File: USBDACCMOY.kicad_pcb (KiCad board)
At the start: 2 copper layers, 49.6 x 77.8 mm, 54 parts, among them CON1 GND_CONNECTORSMD, IC1 OPA2134P, J1 USB, Q1 12MHz, U1 NMA0512SC, U2 PCM2707C

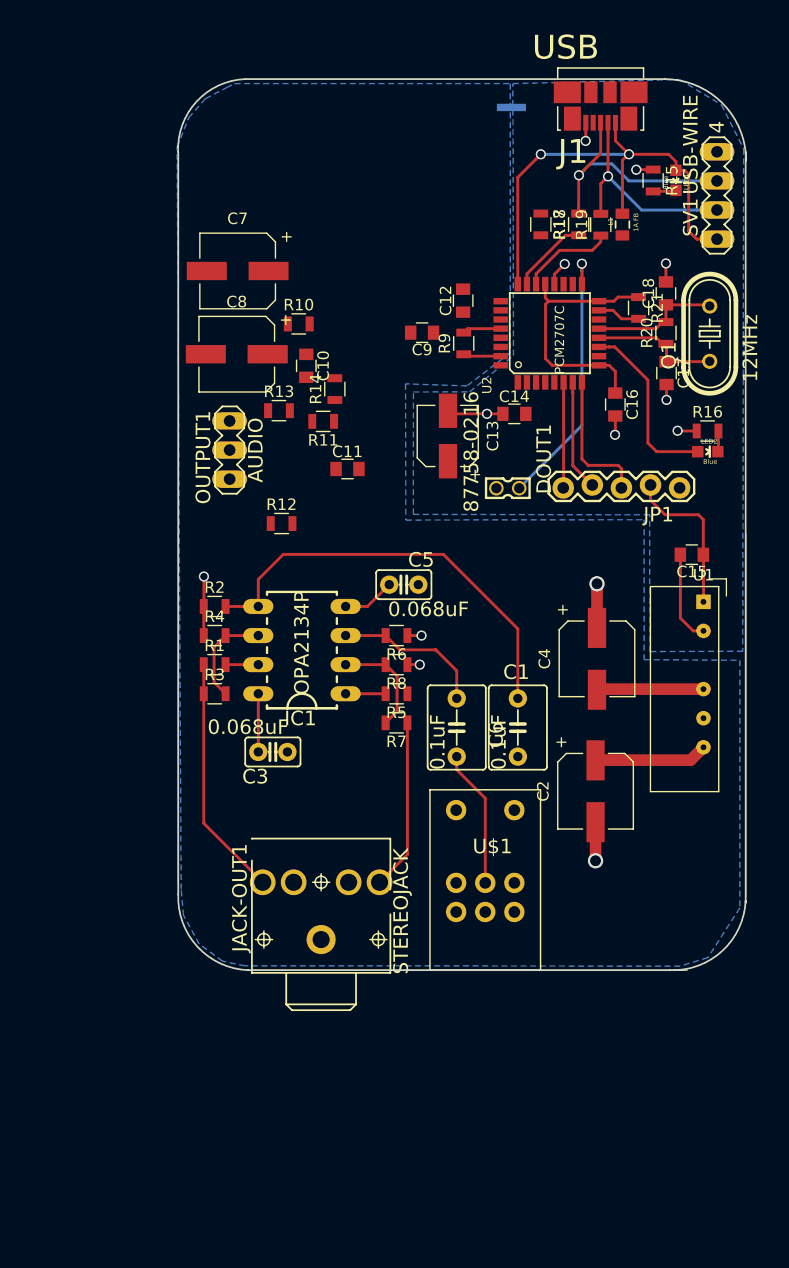
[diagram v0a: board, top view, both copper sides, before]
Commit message: Updated Design Files
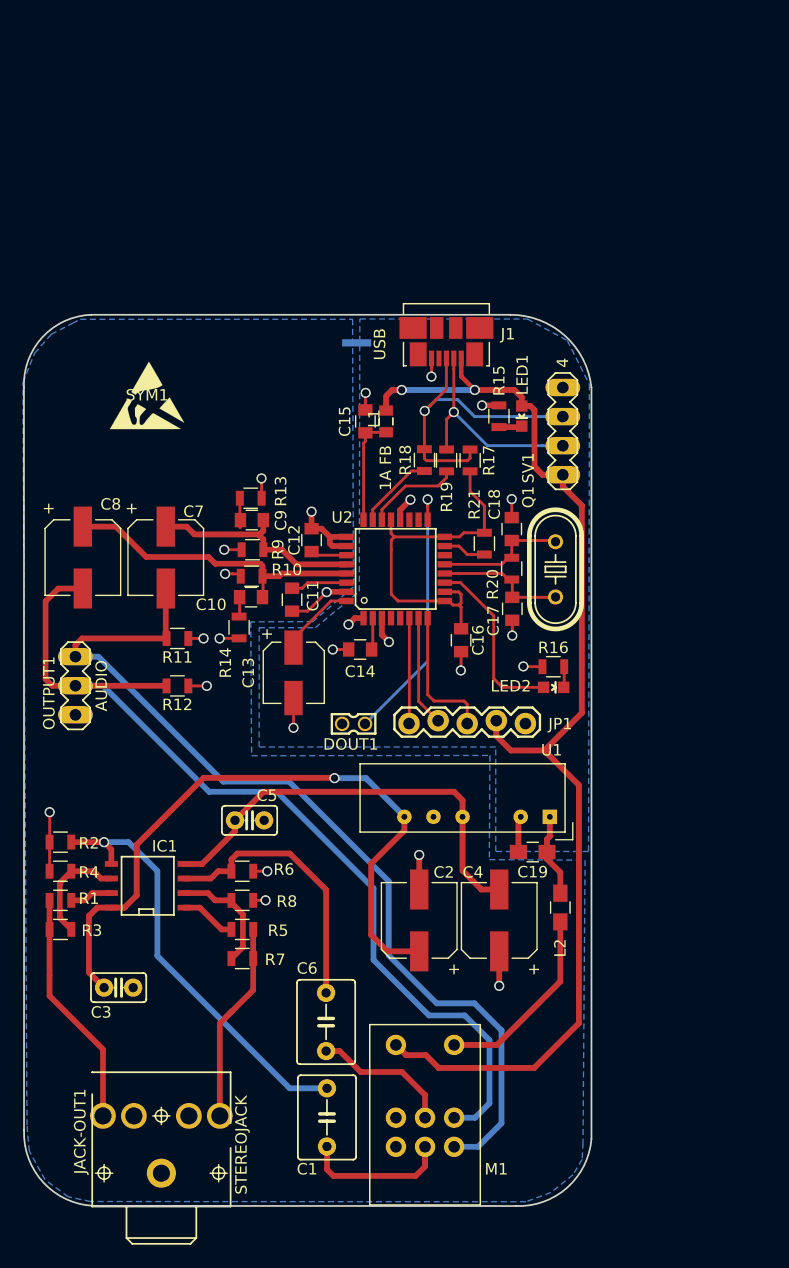
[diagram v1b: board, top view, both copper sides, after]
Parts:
- removed U$1: ~, CMOY:AUDIO-POTS_ALPS_RK0971221Z0X
- added C19: C, Capacitors_SMD:C_0805_HandSoldering, F.Cu at (145.9, 121.4)
- added L2: L, Capacitors_SMD:C_0805_HandSoldering, F.Cu at (148.3, 126.3)
- added M1: AUDIO-POTS_ALPS_RK0971221Z05, PCM2707:AUDIO-POTS_ALPS_RK0971221Z0X, F.Cu at (136.5, 144.6)
- added SYM1: SYM_ESD_Small, Symbols:ESD-Logo_6.6x6mm_SilkScreen, F.Cu at (112.3, 81.5)
- IC1: footprint CMOY:DIL-8 -> SMD_Packages:SOIC-8-N
- moved C1 37.9 mm to (128.0, 144.6)
- moved C15 30.8 mm to (131.3, 83.8), turned to 90 degrees
- moved C6 28.1 mm to (127.9, 136.2)
- moved L1 26.9 mm to (133.1, 83.8)
- moved C7 25.8 mm to (113.9, 95.7), turned to 270 degrees
- moved R9 25.8 mm to (121.5, 95.0), turned to 0 degrees
- moved C12 24.7 mm to (126.6, 94.2)
- moved JACK-OUT1 24.7 mm to (113.4, 152.1)
- moved C13 24.7 mm to (125.0, 105.8), turned to 270 degrees
- moved CON1 24.6 mm to (131.2, 77.0)
- moved C5 24.6 mm to (121.2, 118.6)
- moved J1 24.6 mm to (138.4, 78.3)
- moved LED1 24.6 mm to (145.0, 83.4)
- moved R16 24.6 mm to (147.7, 105.2)
- moved R18 24.6 mm to (136.5, 87.2)
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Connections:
- C15 pad 1: VBUS -> Net-(C15-Pad1)
- L1 pad 1: VBUS -> Net-(C15-Pad1)
- U1 pad 1: VBUS -> Net-(C19-Pad1)
- U2 pad 24: VBUS -> Net-(C15-Pad1)
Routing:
- net INPUT_R: track 0.00 -> 83.1 mm
- net INPUT_L: track 0.00 -> 81.2 mm
- net VBUS: track 56.5 -> 105.3 mm
- net V+: track 15.0 -> 59.6 mm, vias 0 -> 1
- net /PCM2707/N$21: track 0.00 -> 27.8 mm
- net V-: track 13.9 -> 38.4 mm
- net /PCM2707/N$23: track 3.37 -> 26.0 mm
- net AGND: track 17.9 -> 35.3 mm, vias 5 -> 13
- net Net-(L2-Pad1): track 0.00 -> 16.8 mm
- net /CMOY/VOLUME-OUT-L: track 0.00 -> 13.4 mm
- net /CMOY/R+: track 13.4 -> 24.2 mm
- net Net-(C15-Pad1): track 0.00 -> 9.47 mm
- net VDD: track 23.2 -> 31.6 mm
- net Net-(C19-Pad1): track 0.00 -> 7.25 mm
- net /PCM2707/N$4: track 0.00 -> 6.78 mm
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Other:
- board size 49.6 x 77.8 mm -> 49.5 x 77.8 mm
- net class Default: clearance 0.254 -> 0.19
- net class VCC added: clearance 0.19, trace_width 0.512, via_dia 0.889, via_drill 0.635
- rule trace_clearance: 0.254 -> 0.19
- board text added: "DRILL STACK ============================= T1 0.51mm 0.020” (5 holes) T2 0.64mm 0.025” (32 holes) T3 0.81mm 0.032” (10 holes) T4 0.90mm 0.035” (2 holes) T5 1.02mm 0.040” (20 holes) T6 1.50mm 0.059” (5 holes) Total plated holes count 74 ============================="
- board text added: "NOTES: UNLESS OTHERWISE SPECIFIED. 1. SURFACE FINISH: • HASL LEAD-FREE 2. PCB DETAILS: • 2 LAYER • 1.6MM ±0.2. • BLACK • FR4 LAMINATE AND PREPREG TO BE IN ACCORDANCE WITH IPC-4101/23 OR IPC-4101/24 3. COPPER WEIGHT: • 1 OZ APPLIED IN ACCORDANCE WITH IPC-4562. COPPER WEIGHTS ARE TO BE CONSIDERED FINISHED. 4. SILKSCREEN IDENT: • WHITE • TOP SIDE ONLY"
